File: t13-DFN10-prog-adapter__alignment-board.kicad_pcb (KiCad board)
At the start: 2 copper layers, 13.2 x 16.8 mm, 21 parts, among them P3 DFN10

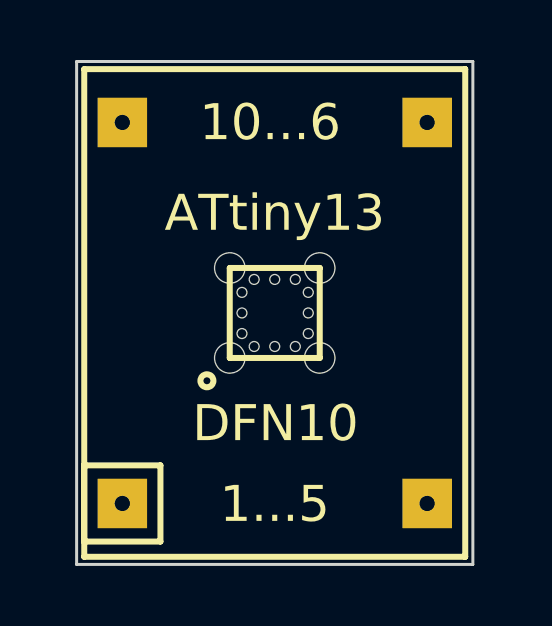
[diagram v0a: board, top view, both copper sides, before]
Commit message: Tweaks.
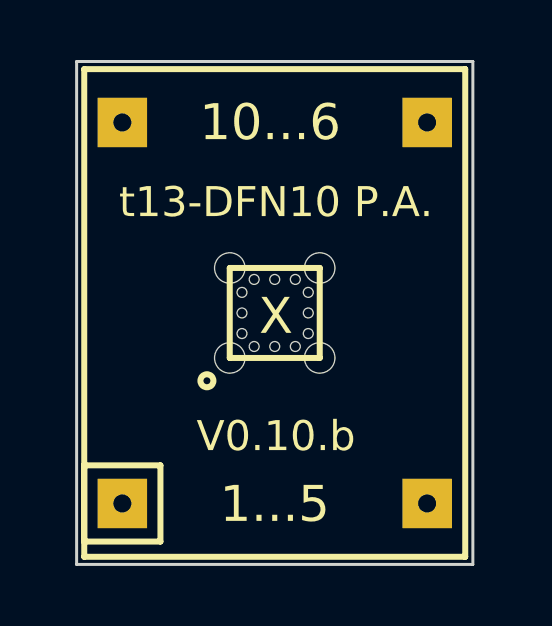
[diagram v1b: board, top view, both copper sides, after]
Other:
- board text added: "V0.10.b"
- board text added: "X"
- board text added: "t13-DFN10 P.A."
- board text removed: "ATtiny13"
- board text removed: "DFN10"
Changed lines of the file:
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@@
-(kicad_pcb (version 3) (host pcbnew "(2014-03-16 BZR 4752)-product")
+(kicad_pcb (version 3) (host pcbnew "(2014-03-14 BZR 4750)-product")
   (general
     (links 0)
@@
     (area 139.15099 91.5068 153.96501 110.7312)
     (thickness 1.6)
-    (drawings 13)
+    (drawings 14)
     (tracks 0)
     (zones 0)
@@
   (page A4)
   (title_block
-    (title "ATtiny13 DFN10 programming adapter")
+    (title "ATtiny13 DFN10 programming adapter - alignment board")
     (date "17 Mar 2014")
-    (rev 0.10.a)
+    (rev 0.10.b)
     (company "2014 - blog.spitzenpfeil.org")
   )
@@
     (mod_text_size 1 1)
     (mod_text_width 0.15)
-    (pad_size 0.3302 0.3302)
-    (pad_drill 0.3302)
+    (pad_size 1.65 1.65)
+    (pad_drill 0.6)
     (pad_to_mask_clearance 0)
     (aux_axis_origin 0 0)
@@
       (effects (font (size 1 1) (thickness 0.2)))
     )
-    (pad 1 thru_hole rect (at 0 0) (size 1.65 1.65) (drill 0.508) (layers *.Cu *.Mask F.SilkS))
+    (pad 1 thru_hole rect (at 0 0) (size 1.65 1.65) (drill 0.6) (layers *.Cu *.Mask F.SilkS))
   )
   (module my_parts:MADW__SIL-1 (layer F.Cu)
@@
       (effects (font (size 1 1) (thickness 0.2)))
     )
-    (pad 1 thru_hole rect (at 0 0) (size 1.65 1.65) (drill 0.508) (layers *.Cu *.Mask F.SilkS))
+    (pad 1 thru_hole rect (at 0 0) (size 1.65 1.65) (drill 0.6) (layers *.Cu *.Mask F.SilkS))
   )
   (module my_parts:MADW__SIL-1 (layer F.Cu)
@@
       (effects (font (size 1 1) (thickness 0.2)))
     )
-    (pad 1 thru_hole rect (at 0 0) (size 1.65 1.65) (drill 0.508) (layers *.Cu *.Mask F.SilkS))
+    (pad 1 thru_hole rect (at 0 0) (size 1.65 1.65) (drill 0.6) (layers *.Cu *.Mask F.SilkS))
   )
   (module my_parts:MADW__SIL-1 (layer F.Cu)
@@
     (fp_line (start 1.27 -1.27) (end 1.27 1.27) (layer F.SilkS) (width 0.2))
     (fp_line (start -1.27 1.27) (end -1.27 -1.27) (layer F.SilkS) (width 0.2))
-    (pad 1 thru_hole rect (at 0 0) (size 1.65 1.65) (drill 0.508) (layers *.Cu *.Mask F.SilkS))
+    (pad 1 thru_hole rect (at 0 0) (size 1.65 1.65) (drill 0.6) (layers *.Cu *.Mask F.SilkS))
+  )
+  (gr_text X (at 146.6 101.2) (layer F.SilkS)
+    (effects (font (size 1.2 1.2) (thickness 0.3)) (justify mirror))
+  )
+  (gr_text V0.10.b (at 146.6 105.2) (layer F.SilkS)
+    (effects (font (size 1 1) (thickness 0.25)))
   )
   (gr_text 10...6 (at 146.4056 94.742) (layer F.SilkS)
@@
   (gr_line (start 153.162 92.71) (end 153.162 109.474) (angle 90) (layer Edge.Cuts) (width 0.1))
   (gr_line (start 139.954 92.71) (end 153.162 92.71) (angle 90) (layer Edge.Cuts) (width 0.1))
-  (gr_text DFN10 (at 146.5834 104.775) (layer F.SilkS)
-    (effects (font (size 1.2 1.2) (thickness 0.25)))
-  )
-  (gr_text ATtiny13 (at 146.558 97.7646) (layer F.SilkS)
-    (effects (font (size 1.2 1.2) (thickness 0.25)))
+  (gr_text "t13-DFN10 P.A." (at 146.6 97.4) (layer F.SilkS)
+    (effects (font (size 1 1) (thickness 0.25)))
   )
   (gr_line (start 140.208 92.964) (end 152.908 92.964) (angle 90) (layer F.SilkS) (width 0.2))
